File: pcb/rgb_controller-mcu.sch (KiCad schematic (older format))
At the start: 23 parts, among them J1 Screw_Terminal_01x04, J2 COM, SW1 SW_Push, SW2 SW_Push, U1 ESP32-WROOM-32D

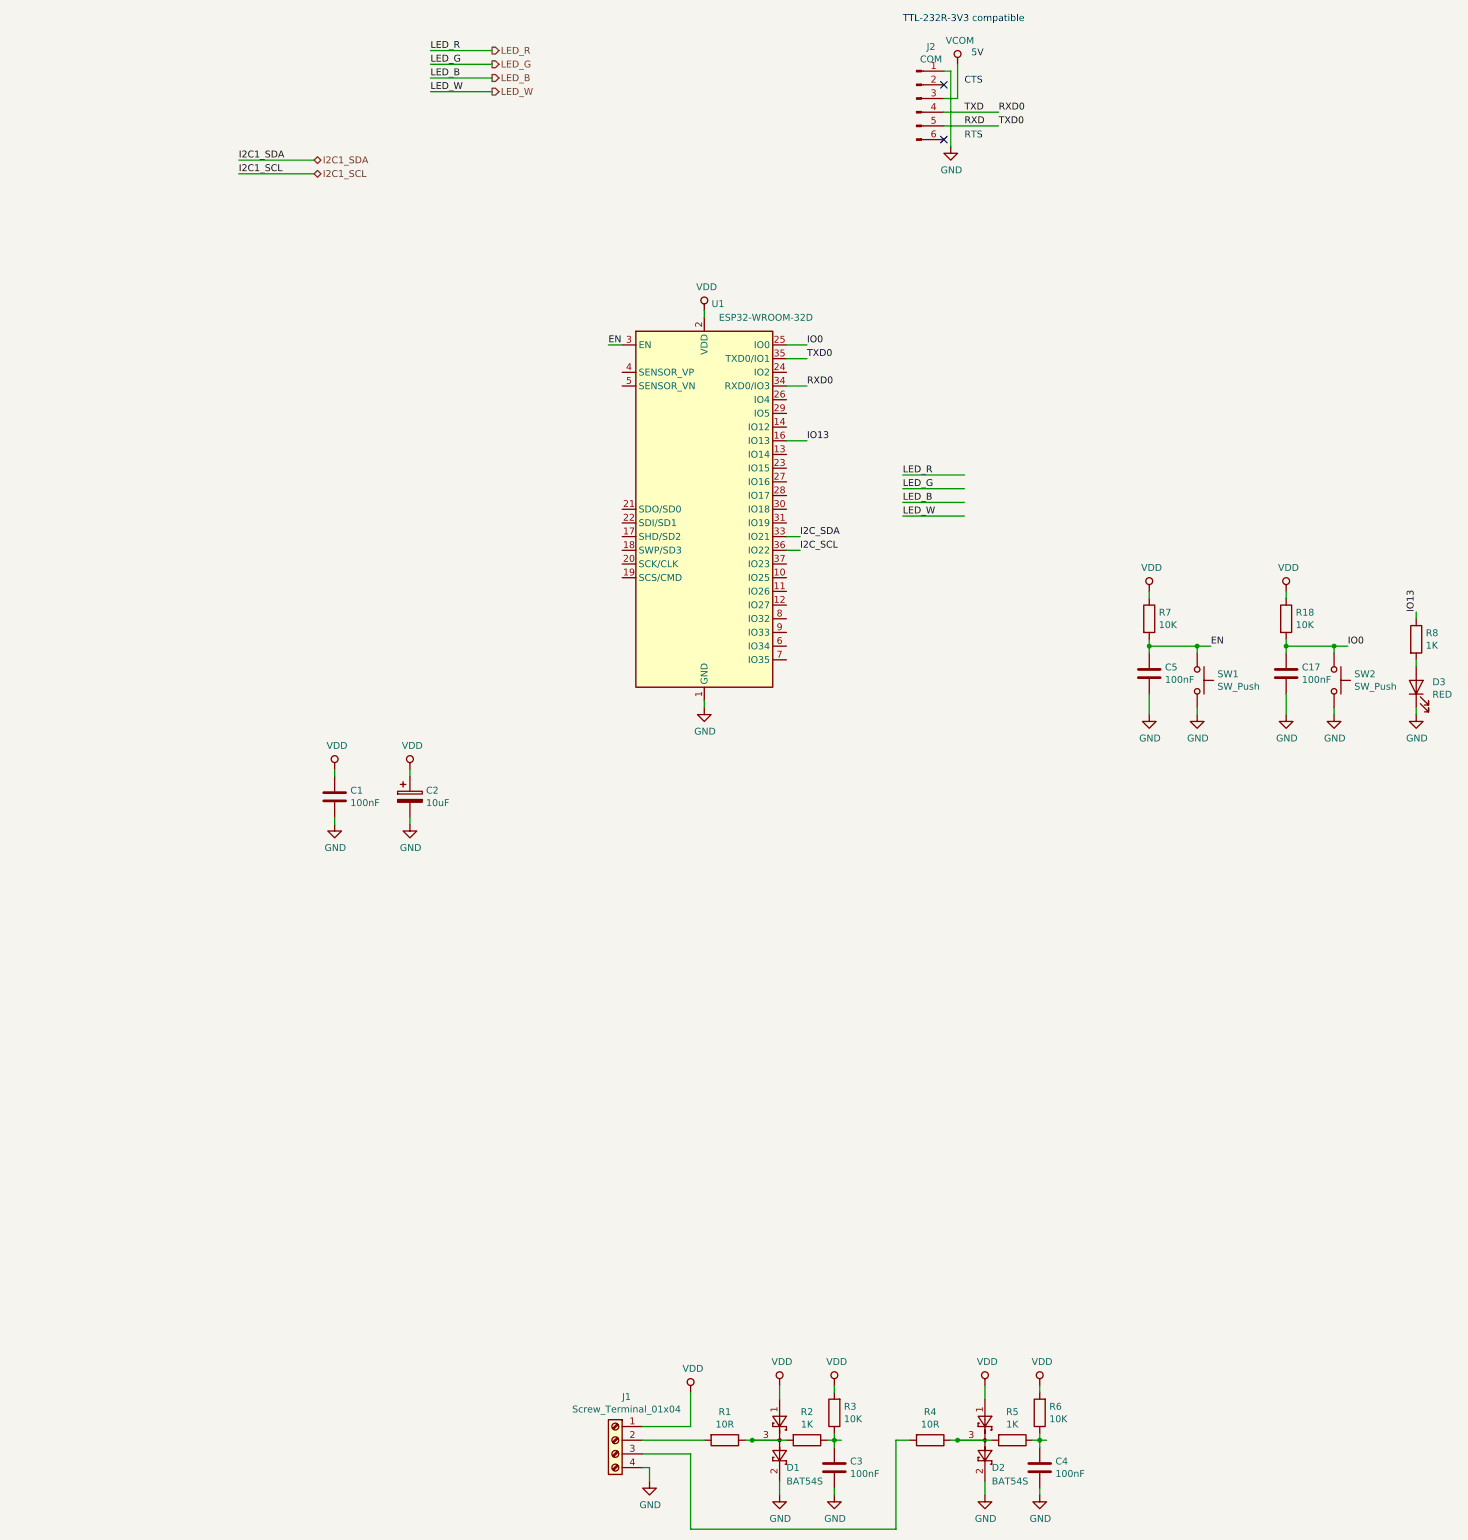
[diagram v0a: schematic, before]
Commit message: backup
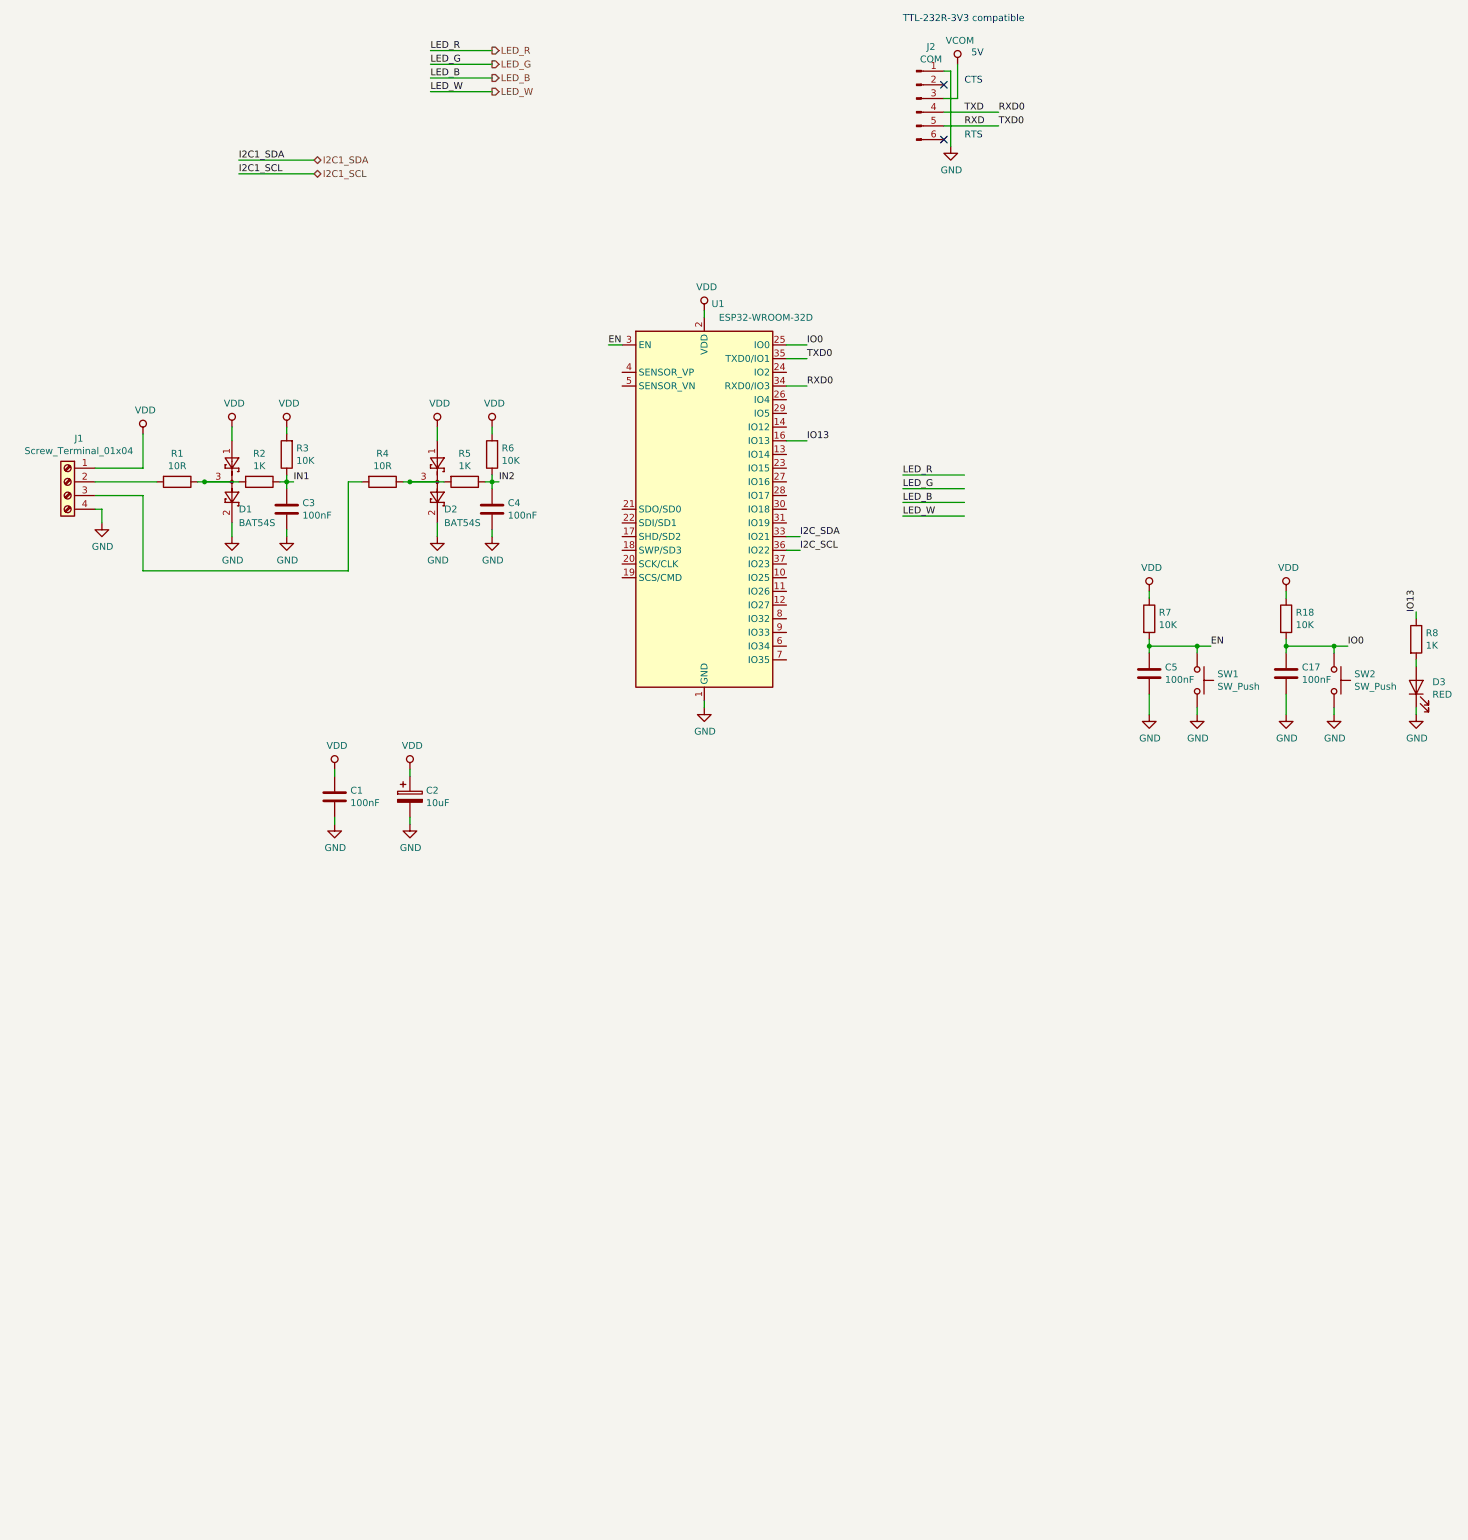
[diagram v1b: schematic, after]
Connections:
- net labels added: IN1, IN2
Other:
- moved on the sheet: C3, C4, D1, D2, J1, R1, R2, R3, R4, R5, R6
